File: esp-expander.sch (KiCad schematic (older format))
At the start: 0 parts

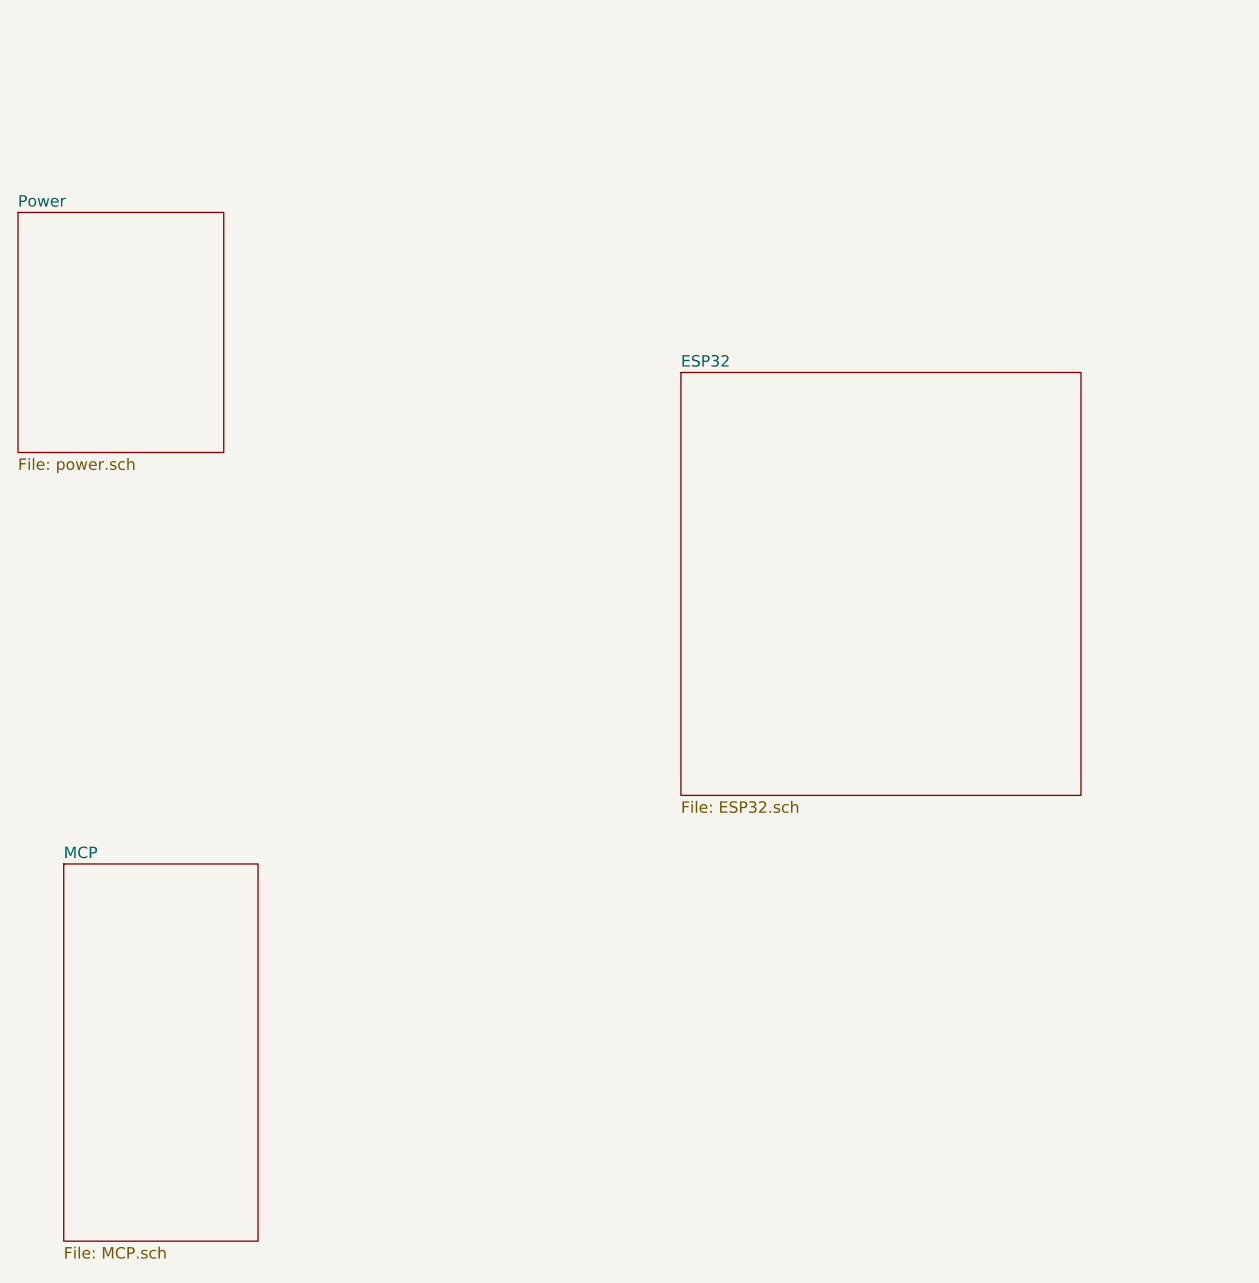
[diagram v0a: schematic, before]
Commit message: Added labels
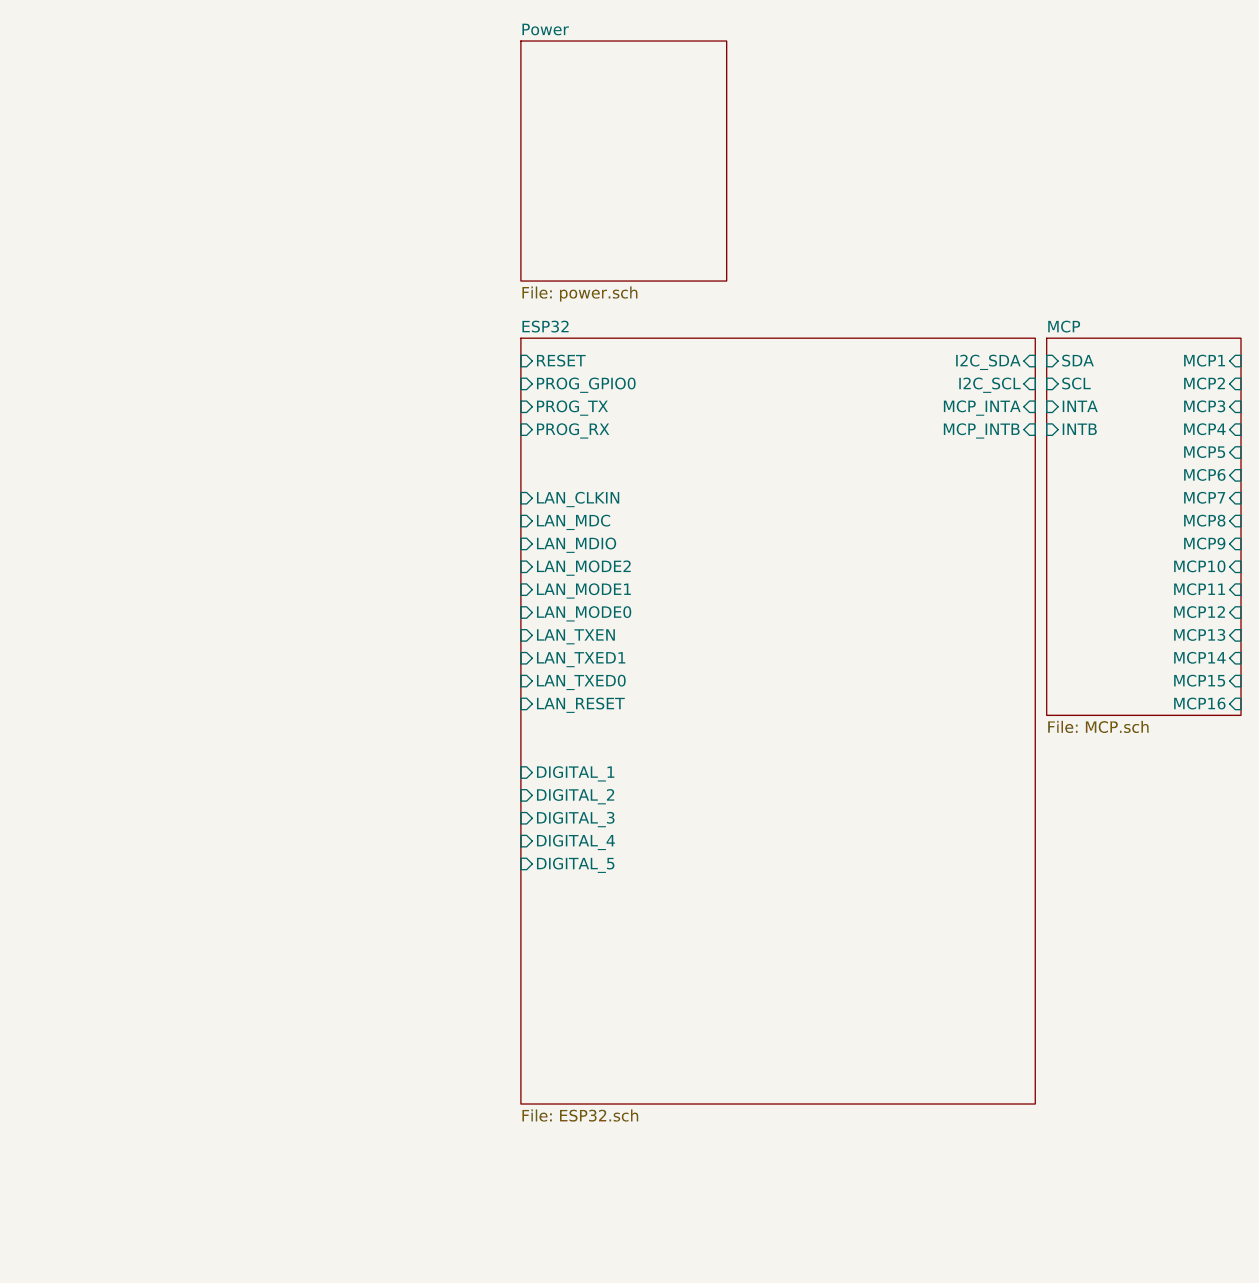
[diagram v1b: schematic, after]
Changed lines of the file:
@@
 $EndDescr
 $Sheet
-S 4950 2700 1750 1850
+S 4250 2550 2250 3350
 U 6212150F
 F0 "ESP32" 50
 F1 "ESP32.sch" 50
+F2 "RESET" I L 4250 2650 50
+F3 "PROG_GPIO0" I L 4250 2750 50
+F4 "PROG_TX" I L 4250 2850 50
+F5 "PROG_RX" I L 4250 2950 50
+F6 "I2C_SCL" I R 6500 2750 50
+F7 "I2C_SDA" I R 6500 2650 50
+F8 "LAN_CLKIN" I L 4250 3250 50
+F9 "LAN_MDC" I L 4250 3350 50
+F10 "LAN_MDIO" I L 4250 3450 50
+F11 "LAN_MODE2" I L 4250 3550 50
+F12 "LAN_MODE1" I L 4250 3650 50
+F13 "LAN_MODE0" I L 4250 3750 50
+F14 "LAN_TXEN" I L 4250 3850 50
+F15 "LAN_TXED1" I L 4250 3950 50
+F16 "LAN_TXED0" I L 4250 4050 50
+F17 "LAN_RESET" I L 4250 4150 50
+F18 "DIGITAL_1" I L 4250 4450 50
+F19 "DIGITAL_2" I L 4250 4550 50
+F20 "DIGITAL_3" I L 4250 4650 50
+F21 "DIGITAL_4" I L 4250 4750 50
+F22 "DIGITAL_5" I L 4250 4850 50
+F23 "MCP_INTA" I R 6500 2850 50
+F24 "MCP_INTB" I R 6500 2950 50
 $EndSheet
 $Sheet
-S 2050 2000 900  1050
+S 4250 1250 900  1050
 U 6213DFD4
 F0 "Power" 50
@@
 $EndSheet
 $Sheet
-S 2250 4850 850  1650
+S 6550 2550 850  1650
 U 6215A73B
 F0 "MCP" 50
 F1 "MCP.sch" 50
+F2 "SDA" I L 6550 2650 50
+F3 "SCL" I L 6550 2750 50
+F4 "INTB" I L 6550 2950 50
+F5 "INTA" I L 6550 2850 50
+F6 "MCP1" I R 7400 2650 50
+F7 "MCP2" I R 7400 2750 50
+F8 "MCP3" I R 7400 2850 50
+F9 "MCP4" I R 7400 2950 50
+F10 "MCP5" I R 7400 3050 50
+F11 "MCP6" I R 7400 3150 50
+F12 "MCP7" I R 7400 3250 50
+F13 "MCP8" I R 7400 3350 50
+F14 "MCP9" I R 7400 3450 50
+F15 "MCP10" I R 7400 3550 50
+F16 "MCP11" I R 7400 3650 50
+F17 "MCP12" I R 7400 3750 50
+F18 "MCP13" I R 7400 3850 50
+F19 "MCP14" I R 7400 3950 50
+F20 "MCP15" I R 7400 4050 50
+F21 "MCP16" I R 7400 4150 50
 $EndSheet
 $EndSCHEMATC
